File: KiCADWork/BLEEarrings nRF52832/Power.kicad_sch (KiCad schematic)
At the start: 10 parts, among them U1 MCP73831T-2ACI/OT, U2 XB6096I2SV

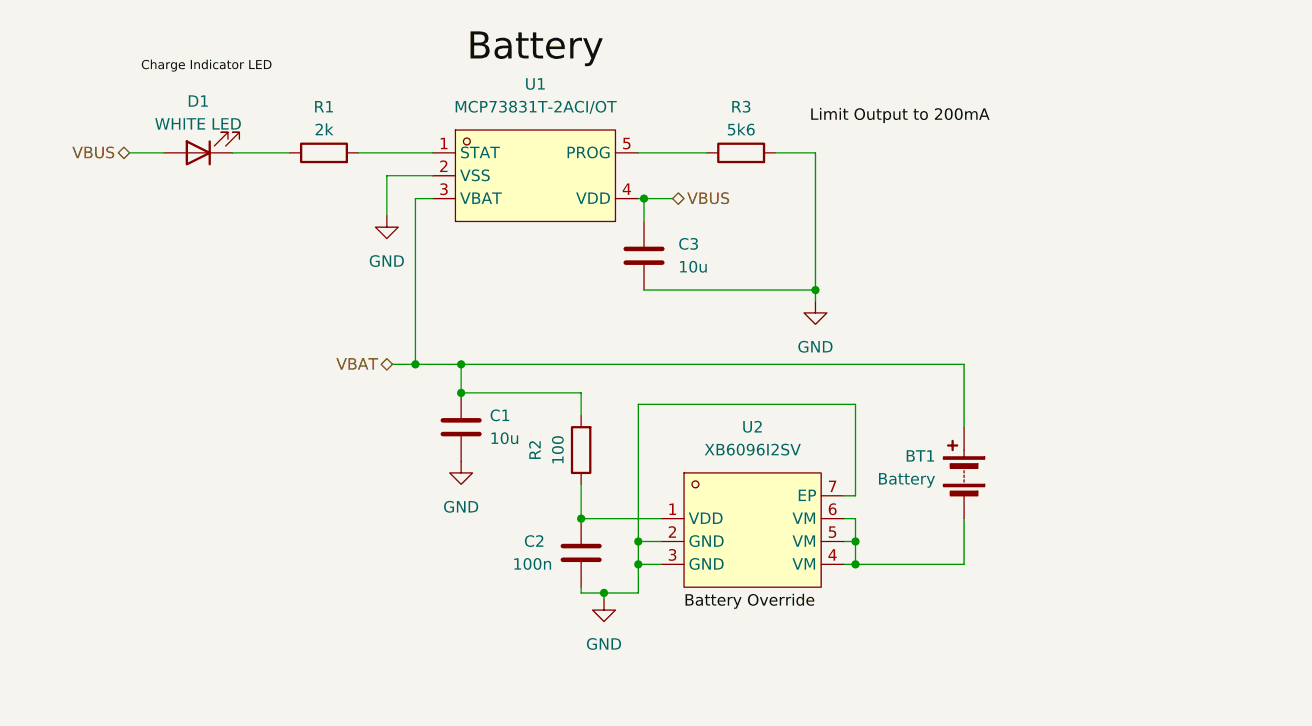
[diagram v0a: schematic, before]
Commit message: Dock Updates
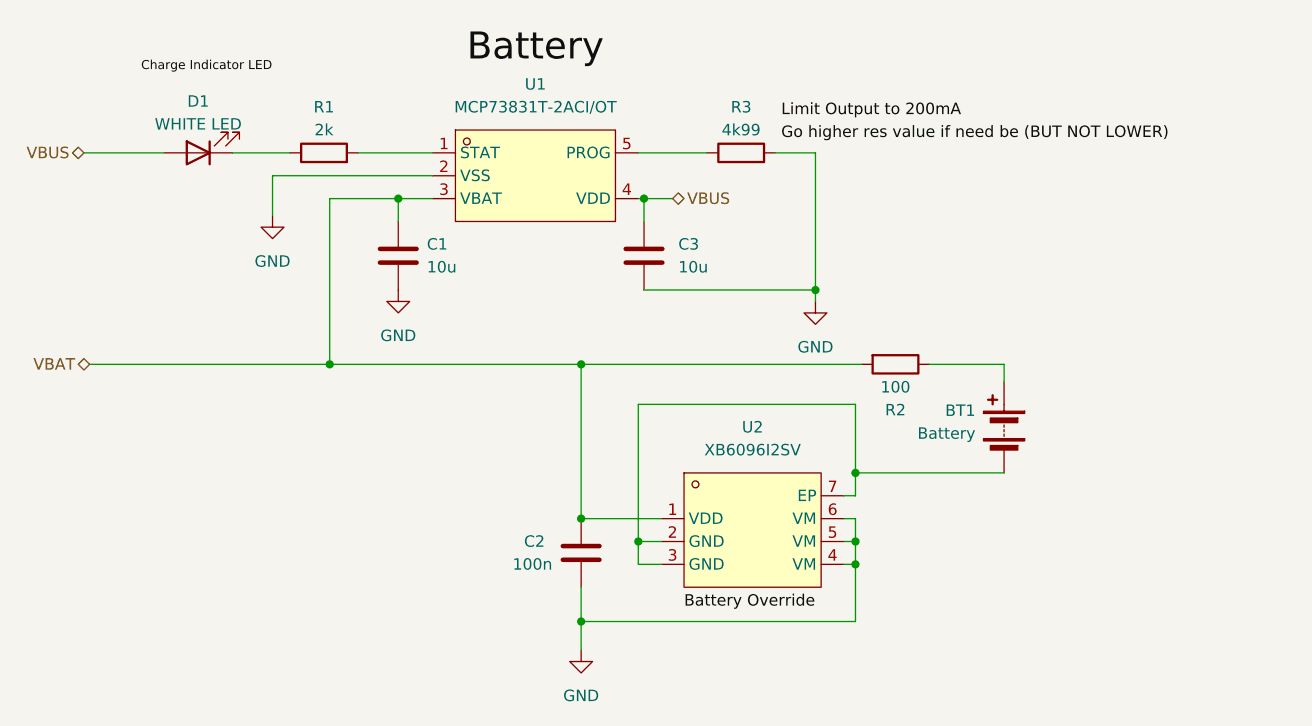
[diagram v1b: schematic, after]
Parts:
- R3: value 5k6 -> 4k99
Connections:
- net GND: now also U2.4 (VM), U2.5 (VM), U2.6 (VM); no longer U2.2 (GND), U2.3 (GND), U2.7 (EP)
- net VBAT: now also C2.1, U2.1 (VDD); no longer BT1.1 (+)
- new net: BT1.2 (-), U2.2 (GND), U2.3 (GND), U2.7 (EP)
- new net: BT1.1 (+), R2.1
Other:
- moved on the sheet: BT1
